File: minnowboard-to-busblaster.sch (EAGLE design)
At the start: 22 parts

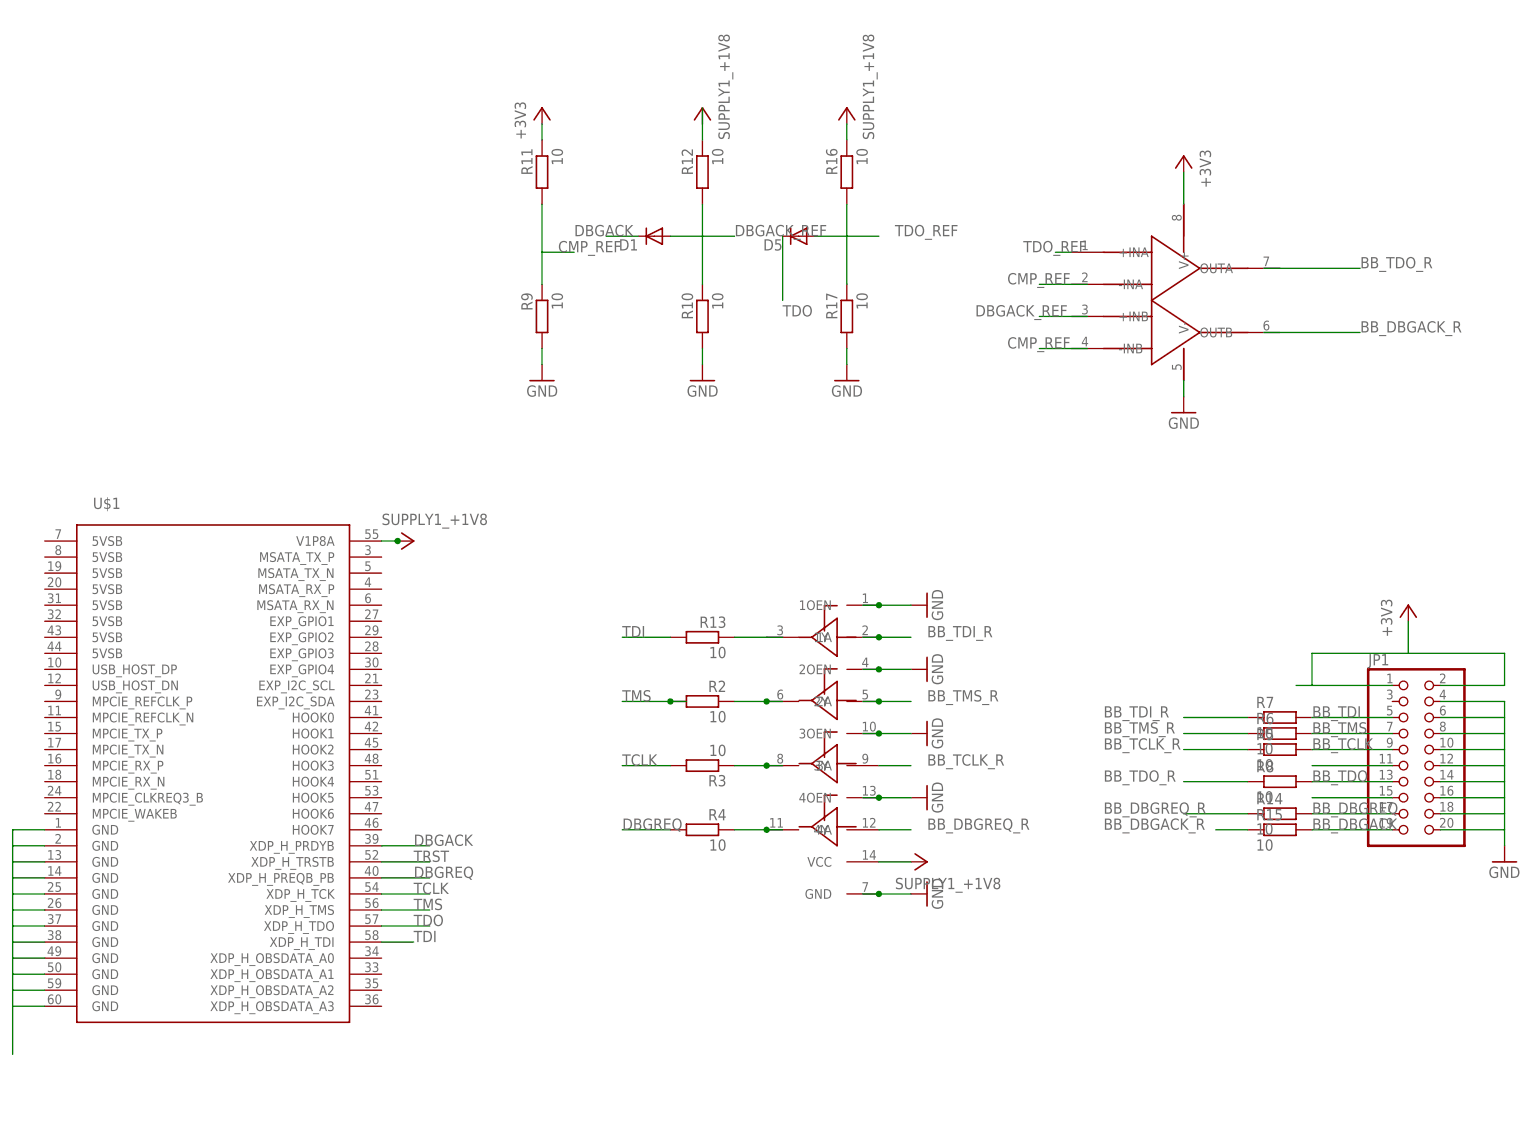
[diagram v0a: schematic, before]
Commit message: all
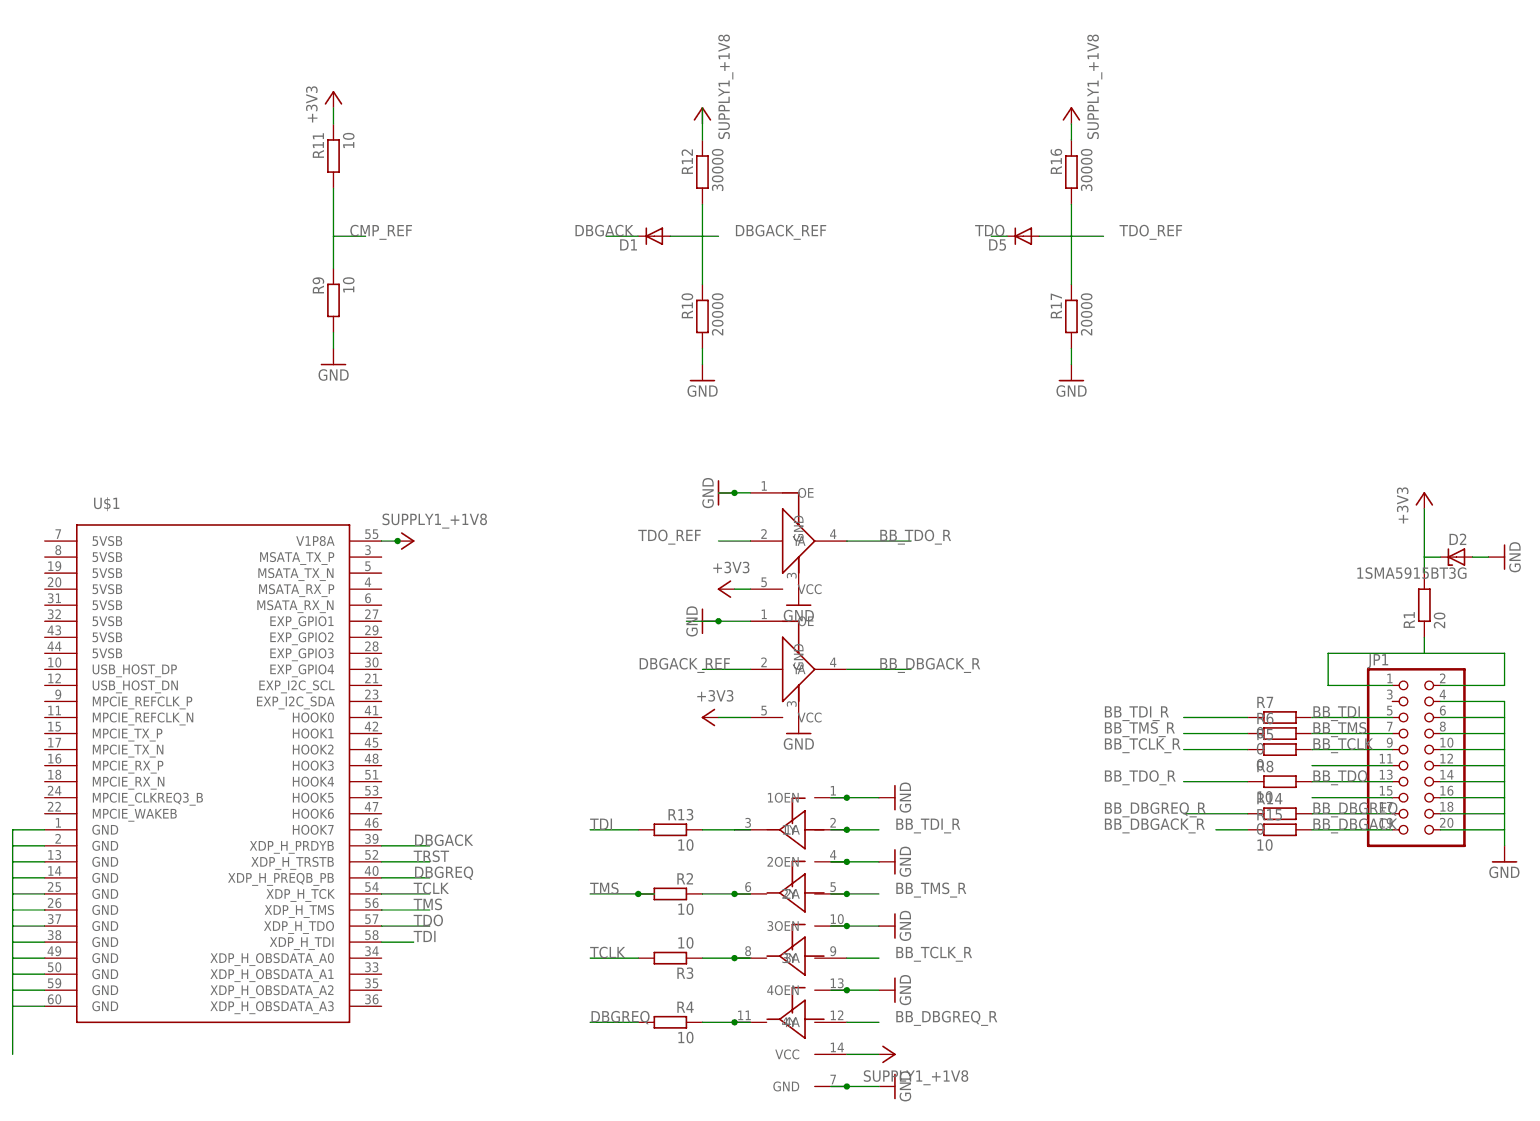
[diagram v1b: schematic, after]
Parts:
- removed U$9: TLV3502-SOT23-8, minnowboard:TLV3502-SOT23-8
- added D2: 1SMA5915BT3G, minnowboard:DIODE_ZENER-DIODESMB
- added R1: 20, resistor:R-EU_R0805
- added U$4, U$6: SN74LV1T125, minnowboard:SN74LV1T125
- R10, R17: value 10 -> 20000
- R12, R16: value 10 -> 30000
- R14, R5, R6, R7: value 10 -> 0
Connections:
- new net N$1: JP1.1, JP1.2, R1.1
- net +3V3: now also D2.C, R1.2, U$4.VCC, U$6.VCC; no longer JP1.1, JP1.2, U$9.V+
- net BB_DBGACK_R: now also U$6.Y
- net BB_TDO_R: now also U$4.Y
- net DBGACK_REF: now also U$6.A
- net GND: now also D2.A, U$4.GND, U$4.OE, U$6.GND, U$6.OE; no longer U$9.V-
- net TDO_REF: now also U$4.A; no longer U$9.+INA
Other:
- moved on the sheet: D5, R11, R13, R16, R17, R2, R3, R4, R9
